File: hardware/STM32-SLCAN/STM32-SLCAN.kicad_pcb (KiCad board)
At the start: 2 copper layers, 29 parts, among them P1 Term, P2 Term, P3 CONN_01X03, P4 CONN_01X04, P5 CONN_01X04, P6 CONN_01X06, U1 MCP2562-I/SN, U2 ISO1050, U3 STM32-BARE

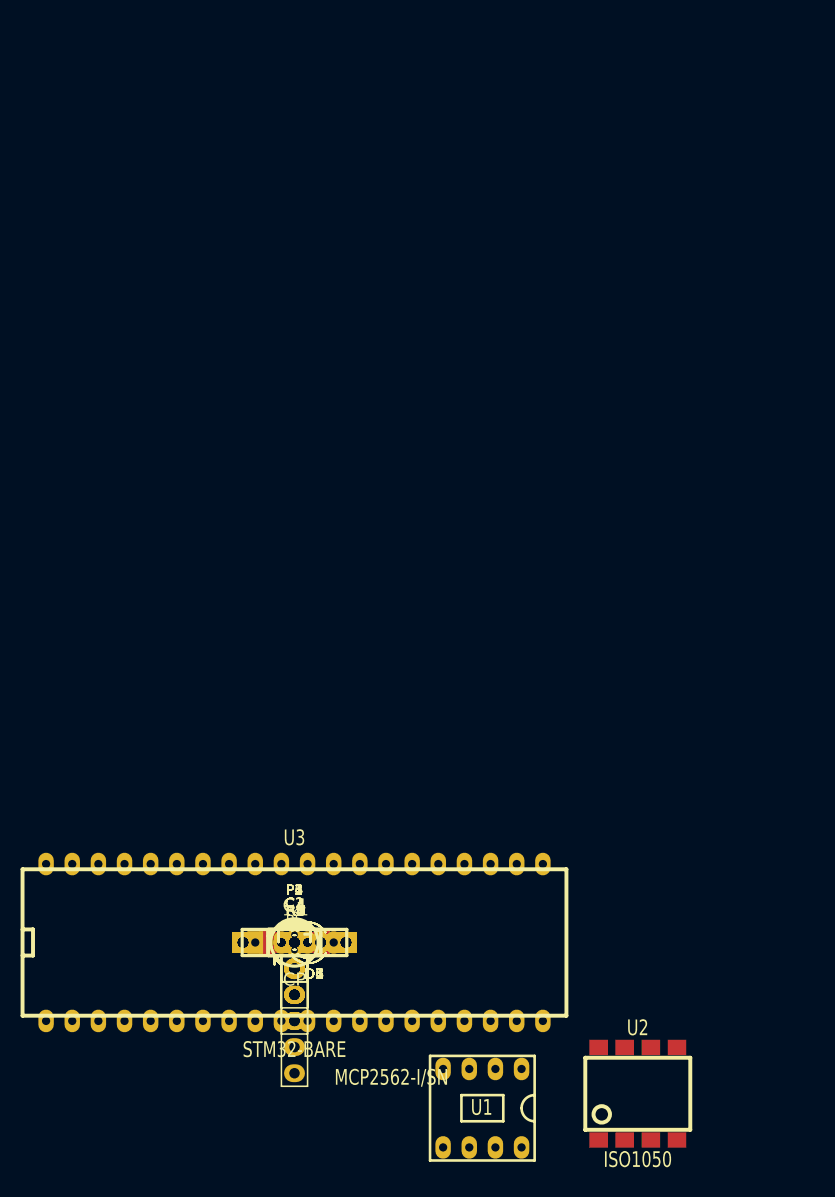
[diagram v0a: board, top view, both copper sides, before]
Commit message: PCB Complete
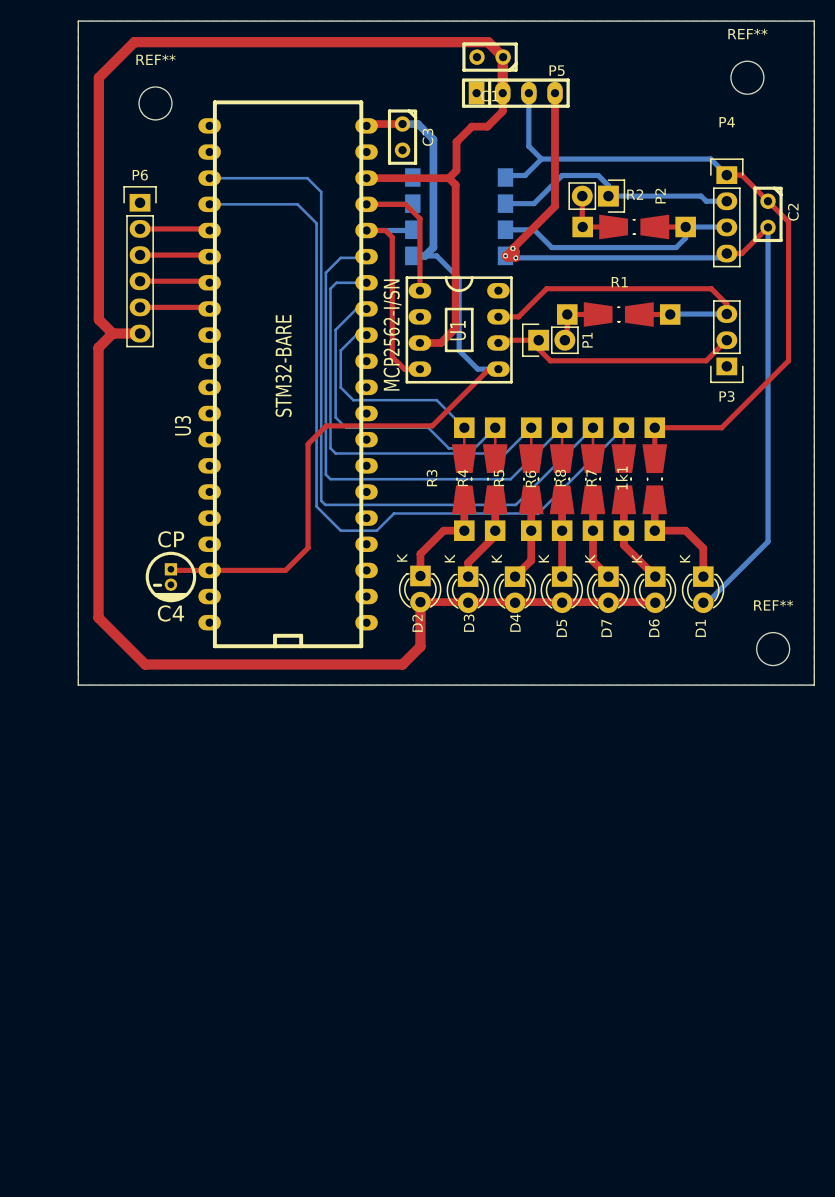
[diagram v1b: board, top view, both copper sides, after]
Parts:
- added REF**: MountingHole_3.2mm_M3, MountingHole:MountingHole_3.2mm_M3, F.Cu at (192.5, 21.0)
- added REF**: MountingHole_3.2mm_M3, MountingHole:MountingHole_3.2mm_M3, F.Cu at (195.0, 76.5)
- added REF**: MountingHole_3.2mm_M3, MountingHole:MountingHole_3.2mm_M3, F.Cu at (135.0, 23.5)
- U2: moved to B.Cu
- moved C1 88.1 mm to (167.5, 19.0), turned to 180 degrees
- moved U2 86.9 mm to (164.5, 34.5), turned to 90 degrees
- moved P4 85.6 mm to (190.5, 30.5)
- moved P5 85.3 mm to (170.0, 22.5)
- moved C2 84.4 mm to (194.5, 34.3), turned to -90 degrees
- moved C3 78.9 mm to (159.0, 26.8), turned to -90 degrees
- moved P2 78.7 mm to (179.0, 32.5), turned to -90 degrees
- moved R2 76.9 mm to (181.5, 35.5)
- moved U1 75.6 mm to (164.5, 45.5), turned to -90 degrees
- moved P6 73.4 mm to (133.5, 33.1)
- moved P3 70.0 mm to (190.5, 49.0), turned to 180 degrees
- moved R1 68.7 mm to (180.0, 44.0)
- moved P1 63.1 mm to (172.2, 46.5), turned to 90 degrees
- moved 1k1 57.0 mm to (183.5, 60.0), turned to 90 degrees
- moved R7 55.2 mm to (180.5, 60.0), turned to 90 degrees
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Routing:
- net +5V: track 0.00 -> 200.3 mm
- net +5VA: track 0.00 -> 84.9 mm, vias 0 -> 3
- net +3V3: track 0.00 -> 82.9 mm
- net /TxD_LED: track 0.00 -> 76.6 mm
- net /RxD_LED: track 0.00 -> 74.1 mm
- net GNDA: track 0.00 -> 69.9 mm
- net /CAN_OVF: track 0.00 -> 52.4 mm
- net /UART_OVF: track 0.00 -> 43.0 mm
- net Net-(P3-Pad3): track 0.00 -> 33.5 mm
- net /CAN_RX: track 0.00 -> 32.9 mm
- net Net-(P4-Pad3): track 0.00 -> 26.7 mm
- net Net-(P1-Pad1): track 0.00 -> 24.5 mm
- net Net-(P2-Pad1): track 0.00 -> 24.3 mm
- net /CAN_TX: track 0.00 -> 23.3 mm
- net Net-(U1-Pad4): track 0.00 -> 22.1 mm
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- added copper zone on B.Cu, net GND
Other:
- board outline added: 71.5 x 64.5 mm
- net class Default removed
